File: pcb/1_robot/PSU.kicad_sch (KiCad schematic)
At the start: 23 parts, among them Q1 NMOS 4A, Q2 NMOS 4A, Q3 NMOS

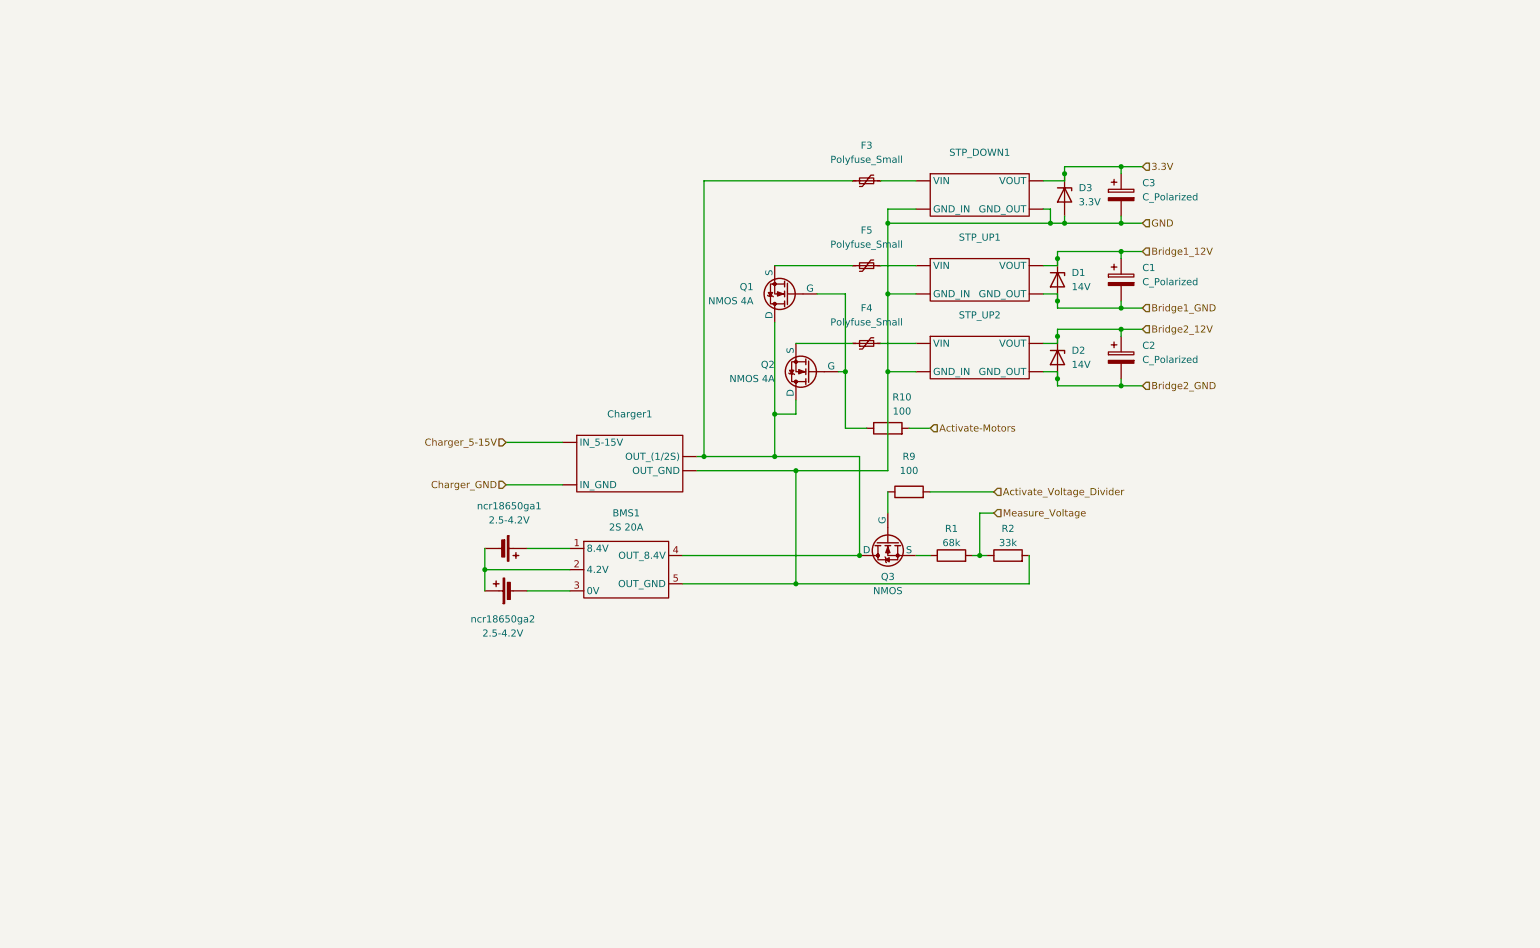
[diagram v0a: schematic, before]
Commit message: finished work
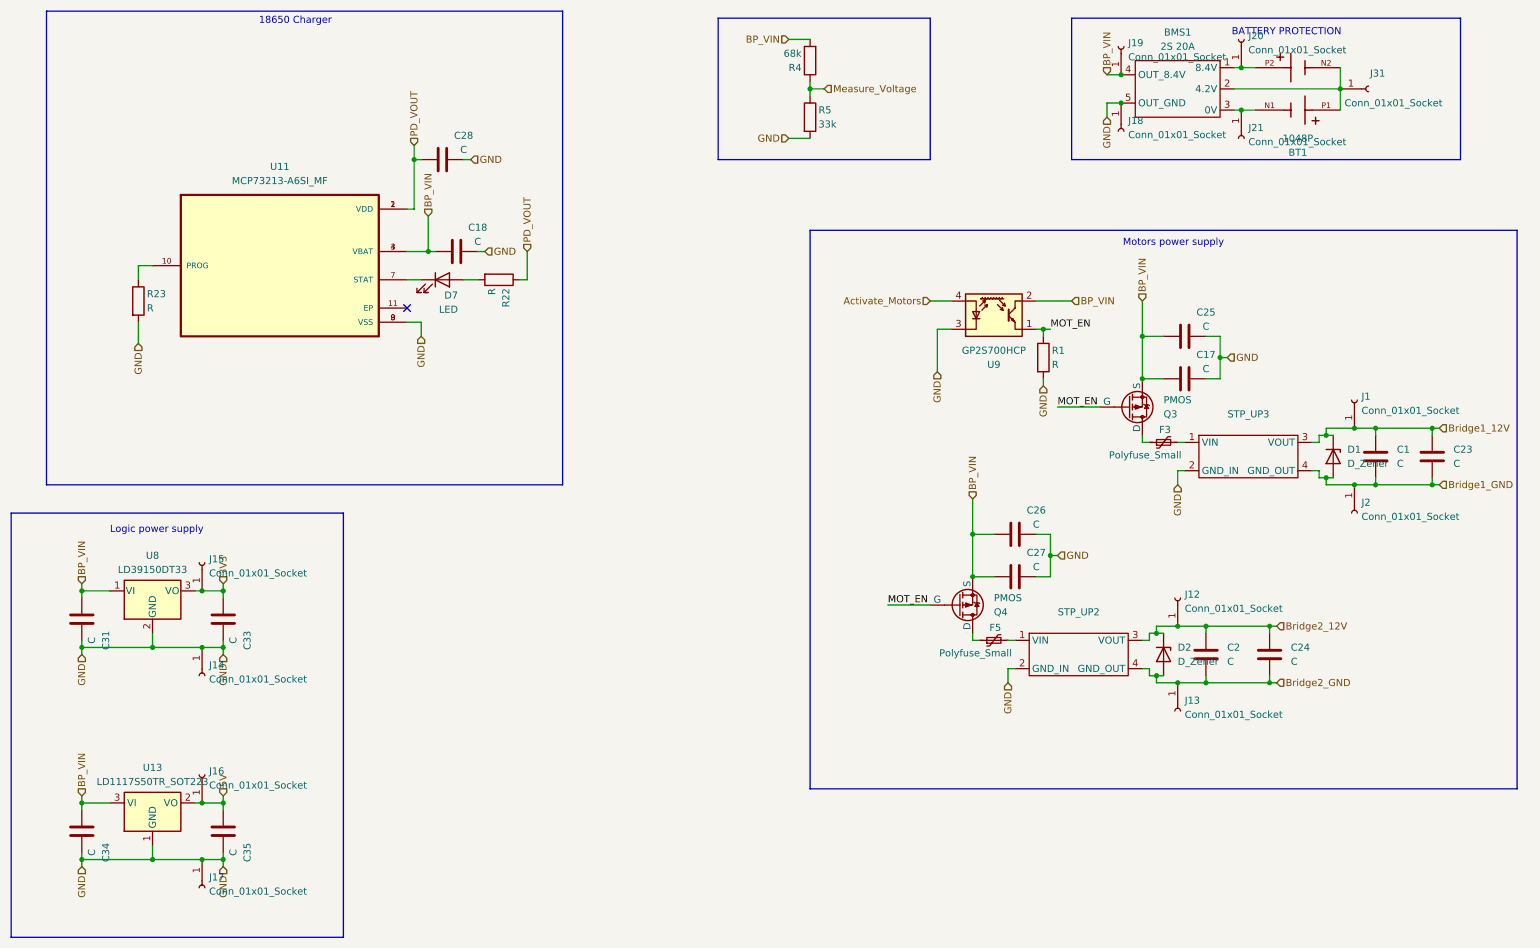
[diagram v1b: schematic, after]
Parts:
- removed C1, C2, C3: C_Polarized, symbol Device:C_Polarized
- removed Charger1: ~, symbol personalized_symbols:TP5100
- removed D3: 3.3V, symbol Device:D_Zener
- removed F4: Polyfuse_Small, symbol Device:Polyfuse_Small
- removed Q1, Q2: NMOS 4A, symbol Simulation_SPICE:NMOS
- removed Q3: NMOS, symbol Simulation_SPICE:NMOS
- removed R10, R9: 100, symbol Device:R
- removed R2: 33k, symbol Device:R
- removed STP_DOWN1: ~, symbol personalized_symbols:Step_down
- removed STP_UP1: ~, symbol personalized_symbols:Step_Up
- removed ncr18650ga1, ncr18650ga2: 2.5-4.2V, symbol Device:Battery_Cell
- added BT1: 1048P, Foot_lib:BAT_1048P, symbol personalized_symbols:1048P
- added C1, C17, C18, C2, C23, C24, C25, C26, C27, C28, C31, C33, C34, C35: C, symbol Device:C
- added D7: LED, symbol Device:LED
- added J1, J12, J13, J2: Conn_01x01_Socket, Connector_PinHeader_2.54mm:PinHeader_1x01_P2.54mm_Vertical, symbol Connector:Conn_01x01_Socket
- added J14, J15, J16, J17, J18, J19, J20, J21, J31: Conn_01x01_Socket, Connector_PinSocket_2.54mm:PinSocket_1x01_P2.54mm_Vertical, symbol Connector:Conn_01x01_Socket
- added Q3, Q4: PMOS, symbol Simulation_SPICE:PMOS
- added R22, R23: R, symbol Device:R
- added R4: 68k, symbol Device:R
- added R5: 33k, symbol Device:R
- added STP_UP3: ~, Foot_lib:H-bridge_SX1308 2A, symbol personalized_symbols:Step_Up
- added U11: MCP73213-A6SI_MF, MCP73213-A6SI_MF:SON50P300X300X100-11N, symbol personalized_symbols:MCP73213-A6SI_MF
- added U13: LD1117S50TR_SOT223, Package_TO_SOT_SMD:SOT-223-3_TabPin2, symbol Regulator_Linear:LD1117S50TR_SOT223
- added U8: LD39150DT33, Package_TO_SOT_SMD:TO-252-3_TabPin2, symbol Regulator_Linear:LD39150DT33
- added U9: GP2S700HCP, OptoDevice:Sharp_GP2S700HCP, symbol Sensor_Proximity:GP2S700HCP
- BMS1: footprint (none) -> Foot_lib:BMS
- D1, D2: value 14V -> D_Zener
- R1: value 68k -> R
- STP_UP2: footprint (none) -> Foot_lib:H-bridge_SX1308 2A
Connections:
- net Bridge1_12V: now also C1.1, C23.1, J1.1 (Pin_1), STP_UP3.3 (VOUT)
- net Bridge1_GND: now also C1.2, C23.2, J2.1 (Pin_1), STP_UP3.4 (GND_OUT)
- net Bridge2_12V: now also STP_UP2.3 (VOUT), C2.1, C24.1, J12.1 (Pin_1); no longer STP_UP2. (VOUT)
- net Bridge2_GND: now also STP_UP2.4 (GND_OUT), C2.2, C24.2, J13.1 (Pin_1); no longer STP_UP2. (VOUT)
- net GND: now also R1.2, STP_UP2.2 (GND_IN), C17.1, C18.1, C25.1, C26.1, C27.1, C28.1, C31.1, C33.1, C34.1, C35.1, J14.1 (Pin_1), J17.1 (Pin_1), J18.1 (Pin_1), R23.2, R5.2, STP_UP3.2 (GND_IN), U11.8 (VSS), U11.9 (VSS), U13.1 (GND), U8.2 (GND), U9.3 (K); no longer STP_UP2. (VOUT)
- net Measure_Voltage: now also R4.1, R5.1; no longer R1.2
- net at F3.1: now also Q3.1 (D); no longer BMS1.4 (OUT_8.4V)
- net at F5.1: now also Q4.1 (D)
- net at F5.2: now also STP_UP2.1 (VIN)
- net at BMS1.1 (8.4V): now also BT1.P2, J20.1 (Pin_1)
- net at BMS1.2 (4.2V): now also BT1.N2, BT1.P1, J31.1 (Pin_1)
- net MOT_EN: now reaches R1.1
- net MOT_EN: now also Q3.2 (G), Q4.2 (G), U9.1
- net at F3.2: now also STP_UP3.1 (VIN)
- net at BMS1.3 (0V): now also BT1.N1, J21.1 (Pin_1)
- new net: R23.1, U11.10 (PROG)
- new net: D7.1 (K), U11.7 (STAT)
- new net: D7.2 (A), R22.2
- new net 3V3: C33.2, J15.1 (Pin_1), U8.3 (VO)
- new net 5V: C35.2, J16.1 (Pin_1), U13.2 (VO)
- new net Activate_Motors: U9.4 (A)
- new net BP_VIN: BMS1.4 (OUT_8.4V), C17.2, C18.2, C25.2, C26.2, C27.2, C31.2, C34.2, J19.1 (Pin_1), Q3.3 (S), Q4.3 (S), R4.2, U11.3 (VBAT), U11.4 (VBAT), U13.3 (VI), U8.1 (VI), U9.2
- new net PD_VOUT: C28.2, R22.1, U11.1 (VDD), U11.2 (VDD)
- no-connect marks 0 -> 1
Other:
- note added: "18650 Charger"
- note added: "BATTERY PROTECTION"
- note added: "Logic power supply"
- note added: "Motors power supply"
- moved on the sheet: BMS1, D2
